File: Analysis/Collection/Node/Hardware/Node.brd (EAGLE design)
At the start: 41.9 x 77.5 mm, 27 parts, among them IC1 4050D, IC2 LP298XS, IC3 DS3231/SO, M2 WIRELESS-NRF24L01-PA-EXT, Q1 16MHz, SW2 FSMSM, U2 ATMEGA328P-PU

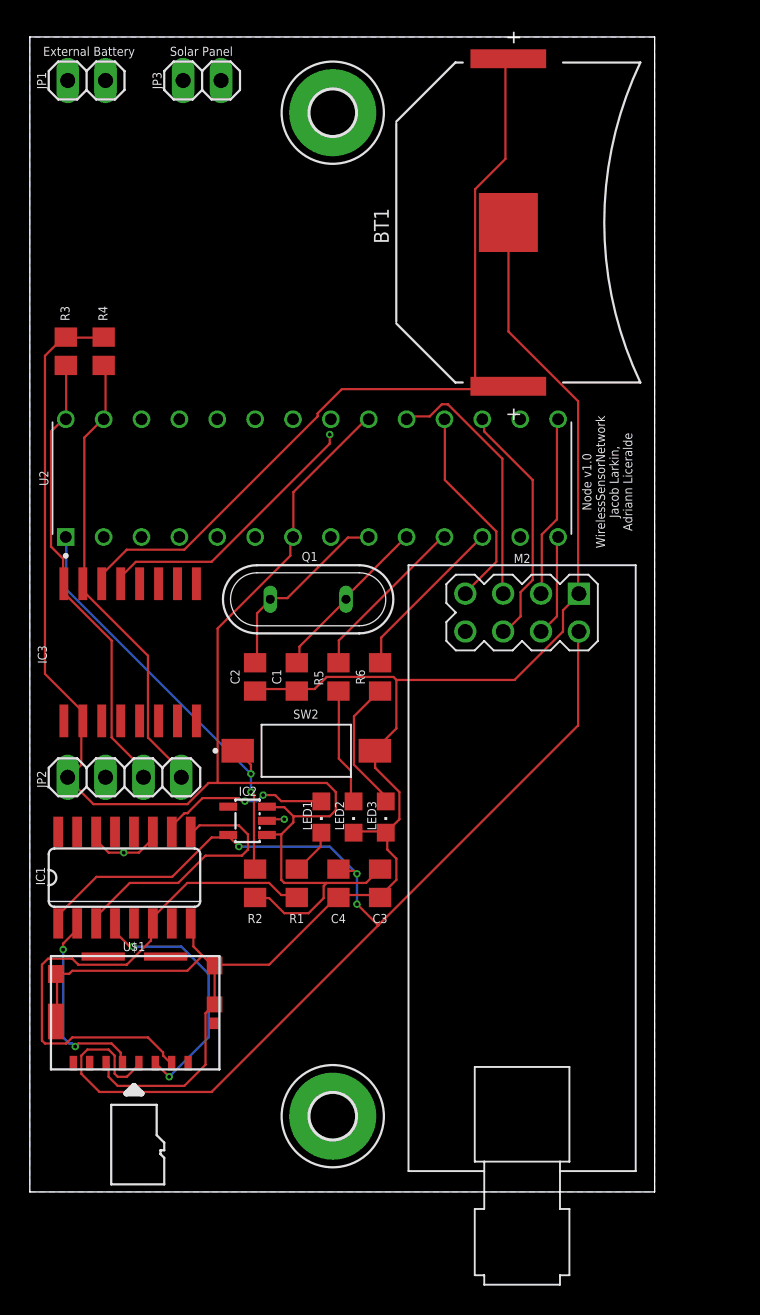
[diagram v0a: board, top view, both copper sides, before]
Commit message: Redesigned Hardware
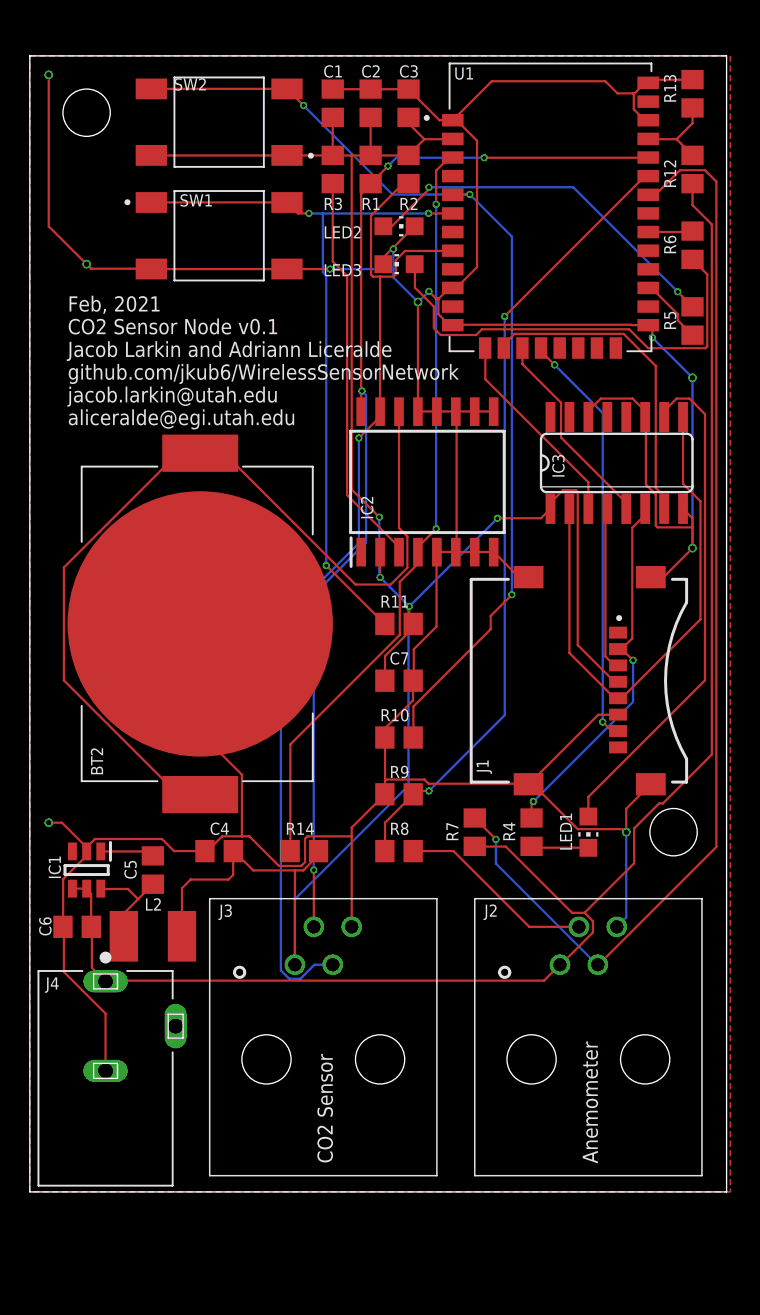
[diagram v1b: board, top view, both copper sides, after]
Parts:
- removed BT1: KEYSTONE_ELECTRONICS_3034KEYSTONE_ELECTRONICS_3034_0_0, Keystone Electronics - 3034:KEYSTONE_ELECTRONICS_3034_0
- removed H1, H2: MOUNT-PAD-ROUND3.0, holes:3,0-PAD
- removed JP1, JP3: (no value), pinhead:1X02
- removed JP2: (no value), pinhead:1X04
- removed M2: WIRELESS-NRF24L01-PA-EXT, diy-modules:WIRELESS-NRF24L01-PA-EXT
- removed Q1: 16MHz, special:QS
- removed U$1: 1051620001A, Molex_micro_SD:1051620001_SMT
- removed U2: ATMEGA328P-PU, Microcontroller:DIP-28
- added BT2: BAT-HLD-001, BAT-HLD-001:BAT_BAT-HLD-001
- added C5: .1 uF, rcl:C0805
- added C6: 2.2 uF, rcl:C0805
- added C7: 1 uF, rcl:C0805
- added J1: MEM2067-02-180-00-A_REVB, MEM2067-02-180-00-A_REVB:GCT_MEM2067-02-180-00-A_REVB
- added J2, J3: 95501-2441, SamacSys_Parts:955012441
- added J4: PJ-102A, PJ-102A:CUI_PJ-102A
- added L2: 12 uH, rcl:L1812
- added R10, R11, R12, R13, R14, R7, R8, R9: 10 K, rcl:R0805
- added SW1: FSM4JSMA, Switch:FSM4JSMA
- added U1: XB3-24Z8UM-J, XB3-24Z8UM-J:XCVR_XB3-24Z8UM-J
- C1: value 22pF -> 8.2 pF
- C2: value 22pF -> 1 uF
- C3: value .1uF -> 10 uF
- C4: value .1uF -> 22 uF
- IC1: value 4050D -> TPS560430X3FDBVR; device 40xx:SO16 -> SamacSys_Parts:SOT95P280X145-6N
- IC2: value LP298XS -> DS3231SN; device adafruit:SOT23-5L -> SamacSys_Parts:SOIC127P1032X265-16N
- IC3: value DS3231/SO -> 4050D; device adafruit:SO16W -> 40xx:SO16
- LED1: value RED -> (none); device led:CHIPLED_0805 -> led:CHIP-LED0805
- LED2: value GREEN -> (none); device led:CHIPLED_0805 -> led:CHIP-LED0805
- LED3: value Yellow -> (none); device led:CHIPLED_0805 -> led:CHIP-LED0805
- R1: value 1K -> 10 K
- R2, R3: value 10K -> 10 K
- R4: value 10K -> 160
- R5, R6: value 1K -> 160
- SW2: value FSMSM -> FSM4JSMA; device Switch:FSMSM -> Switch:FSM4JSMA
- moved C3 52.4 mm to (25.4, 73.0), turned to 90 degrees
- moved R2 49.0 mm to (25.4, 68.6), turned to 90 degrees
- moved R1 48.1 mm to (22.9, 68.6)
- moved R4 43.2 mm to (33.7, 24.1)
- moved SW2 42.6 mm to (12.7, 71.8), turned to 270 degrees
- moved LED2 39.7 mm to (24.8, 64.8), turned to 270 degrees
- moved C2 39.3 mm to (22.9, 73.0), turned to 90 degrees
- moved C1 38.6 mm to (20.3, 73.0), turned to 90 degrees
- moved LED3 37.1 mm to (24.8, 62.2), turned to 90 degrees
- moved R6 35.7 mm to (44.5, 63.5), turned to 270 degrees
- moved IC3 35.0 mm to (39.4, 48.9)
- moved R5 33.7 mm to (44.5, 58.4)
- moved IC2 25.7 mm to (26.7, 47.6)
- moved R3 21.7 mm to (20.3, 68.6)
- moved LED1 17.9 mm to (37.5, 24.1)
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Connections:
- removed net +5V: C3.1, IC2.1, IC2.3, IC3.2, JP2.4, R2.2, R3.2, R4.2, U2.20, U2.7
- removed net 32KHZ: IC3.1
- removed net CE: M2.3, U2.15
- removed net CLK: IC1.3, IC1.9
- removed net CS: IC1.7
- removed net CSN: M2.4, U2.14
- removed net DI: IC1.5
- removed net DO: U$1.7
- removed net N$7: C1.1, Q1.1, U2.10
- removed net SCK: M2.5, U2.19
- removed net SQW: IC3.3
- removed net VBAT: BT1.2, BT1.2-2, IC3.14
- removed net V_PACK: JP1.1
- new net !INT: IC2.3, R3.1
- new net !SS: IC3.7, U1.14
- new net ANEM_DIR: J2.2, R8.2
- new net ANEM_DIR/2: R8.1, R9.2, U1.29
- new net ANEM_SPD: J2.3, R7.1, U1.28
- new net N$13: R6.1, U1.26
- new net N$14: R11.1, SW1.1, SW1.2, U1.6
- new net N$16: R10.2, SW2.3, SW2.4, U1.5
- new net SCLK: IC3.3, U1.13
- new net VCC: C6.1, IC1.4, IC1.5, J2.1, J4.1, R12.2, R7.2
- new net VCC/2: R12.1, R13.2, U1.31
- net !RTC_RST: now also IC2.4, R14.1, U1.3; no longer IC3.4
- net +3V3: now also C1.1, C2.1, C3.1, C7.1, IC2.2, IC3.1, J1.4, J3.1, L2.1, R1.2, R11.2, R14.2, R2.2, R3.2, SW2.1, SW2.2, U1.2; no longer IC1.1, IC2.5, M2.2, U$1.4
- net GND: now also BT2.N1, C6.2, C7.2, IC1.2, IC2.10, IC2.11, IC2.12, IC2.13, IC2.5, IC2.6, IC2.7, IC2.8, IC2.9, IC3.11, IC3.14, IC3.8, J1.10, J1.11, J1.12, J1.6, J1.9, J2.4, J3.4, J4.2, R10.1, R13.1, R9.1, SW1.3, SW1.4, U1.1, U1.10, U1.12, U1.21, U1.32, U1.34; no longer BT1.1, IC1.11, IC1.14, IC1.8, IC2.2, IC3.13, JP1.2, JP2.3, JP3.2, M2.1, SW2.2, U$1.6, U$1.G1, U$1.G2, U$1.G3, U$1.G4, U2.21, U2.22, U2.8
- net MISO: now also J1.7, U1.16; no longer M2.7, U2.18
- net MOSI: now also IC3.5, U1.15; no longer M2.6, U2.17
- net N$1: now also LED2.A, R5.2; no longer IC1.10, LED1.A
- net N$10: now also LED1.C, R4.1; no longer LED2.A, R5.1
- net N$11: now also IC3.2, IC3.9, J1.5; no longer LED3.A, R6.1
- net N$12: now also R5.1, U1.23; no longer R6.2, U2.12
- net N$2: now also IC3.4, J1.3; no longer IC1.2, U$1.5
- net N$3: now also C5.2, IC1.1; no longer IC1.6, R1.1, U$1.2
- net N$4: now also BT2.P1, BT2.P2, IC2.14; no longer LED1.C, R1.2
- net N$5: now also C5.1, IC1.6, L2.2; no longer IC1.4, U$1.3
- net N$6: now also IC3.6, J1.2, R4.2; no longer R2.1, SW2.1, U2.1
- net N$8: now also LED3.A, R6.2; no longer C2.1, Q1.2, U2.9
- net N$9: now also IC3.10, LED1.A; no longer R5.2, U2.11
- net SCL: now also IC2.16, J3.2, R1.1, U1.30; no longer IC3.16, JP2.2, R3.1, U2.28
- net SDA: now also IC2.15, J3.3, R2.1, U1.8; no longer IC3.15, JP2.1, R4.1, U2.27
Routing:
- net GND: track 142.8 -> 290.6 mm, vias 3 -> 11
- net +5V: track 108.1 -> 0.00 mm
- net VCC: track 0.00 -> 105.7 mm
- net ANEM_SPD: track 0.00 -> 74.7 mm, vias 0 -> 1
- net N$16: track 0.00 -> 65.8 mm, vias 0 -> 3
- net VBAT: track 58.6 -> 0.00 mm
- net +3V3: track 87.0 -> 145.1 mm, vias 3 -> 4
- net N$4: track 3.15 -> 61.0 mm
- net ANEM_DIR/2: track 0.00 -> 53.2 mm, vias 0 -> 2
- net !RTC_RST: track 0.00 -> 51.2 mm, vias 0 -> 2
- net N$14: track 0.00 -> 49.8 mm, vias 0 -> 3
- net SCL: track 30.7 -> 72.5 mm, vias 0 -> 4
- net SDA: track 31.1 -> 67.6 mm, vias 0 -> 1
- net N$3: track 35.9 -> 3.63 mm
- net N$11: track 9.08 -> 36.0 mm
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- added copper zone on layer 1, net GND
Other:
- board size 41.9 x 77.5 mm -> 46.7 x 76.2 mm
- board text added: "Anemometer"
- board text added: "CO2 Sensor"
- board text added: "Feb, 2021 CO2 Sensor Node v0.1 Jacob Larkin and Adriann Liceralde github.com/jkub6/WirelessSensorNetwork jacob.larkin@utah.edu aliceralde@egi.utah.edu"
- board text removed: "External Battery"
- board text removed: "Node v1.0 WirelessSensorNetwork Jacob Larkin, Adriann Liceralde"
- board text removed: "Solar Panel"
